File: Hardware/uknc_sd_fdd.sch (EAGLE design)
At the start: 21 parts, among them U1 USD-SOCKET

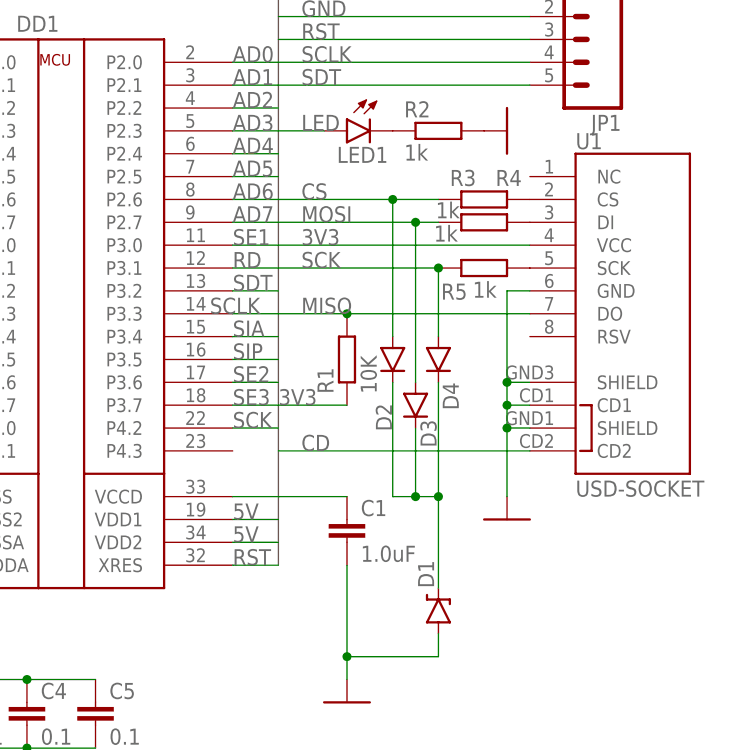
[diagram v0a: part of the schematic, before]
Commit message: исправлена схема
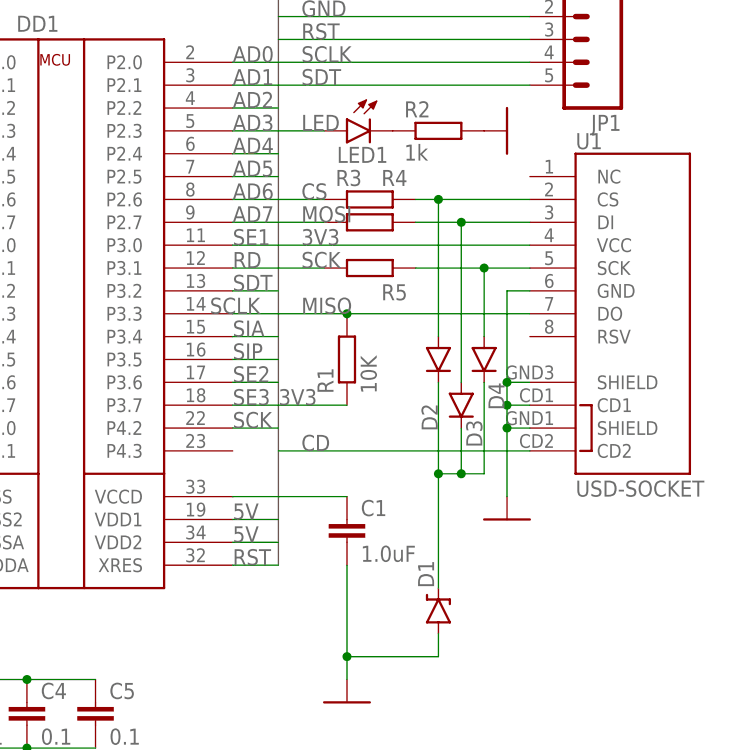
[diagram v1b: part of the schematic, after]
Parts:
- R3, R4, R5: value 1k -> (none)
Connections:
- net CS: no longer D2.A
- net MOSI: no longer D3.A
- net N$4: now also D2.A, R3.2, U1.CS; no longer R5.2, U1.SCK
- net N$5: now also D3.A
- net N$6: now also D4.A, R5.2, U1.SCK; no longer R3.2, U1.CS
- net SCK: no longer D4.A
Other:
- moved on the sheet: D2, D3, D4, R3, R4, R5
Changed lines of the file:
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@@
 <setting verticaltext="up"/>
 </settings>
-<grid distance="0.1" unitdist="inch" unit="inch" style="lines" multiple="1" display="no" altdistance="0.000000123031" altunitdist="inch" altunit="inch"/>
+<grid distance="0.1" unitdist="inch" unit="inch" style="lines" multiple="1" display="no" altdistance="0.01" altunitdist="inch" altunit="inch"/>
 <layers>
 <layer number="1" name="Top" color="4" fill="1" visible="no" active="no"/>
@@
 <part name="C5" library="resistor" deviceset="C-EU" device="C0805" value="0.1"/>
 <part name="C6" library="resistor" deviceset="CPOL-EU" device="E1.8-4" value="10.0"/>
-<part name="R3" library="resistor" deviceset="R-EU_" device="R0805" value="1k"/>
-<part name="R4" library="resistor" deviceset="R-EU_" device="R0805" value="1k"/>
-<part name="R5" library="resistor" deviceset="R-EU_" device="R0805" value="1k"/>
+<part name="R3" library="resistor" deviceset="R-EU_" device="R0805"/>
+<part name="R4" library="resistor" deviceset="R-EU_" device="R0805"/>
+<part name="R5" library="resistor" deviceset="R-EU_" device="R0805"/>
 </parts>
 <sheets>
@@
 <instance part="JP1" gate="G$1" x="132.08" y="91.44" rot="R180"/>
 <instance part="U$8" gate="G$1" x="121.92" y="38.1"/>
-<instance part="D2" gate="G$1" x="109.22" y="55.88" smashed="yes" rot="R270">
-<attribute name="NAME" x="107.35603125" y="50.992" size="1.778" layer="95" rot="R270"/>
-<attribute name="VALUE" x="106.9086" y="53.34" size="1.778" layer="96" rot="R270"/>
+<instance part="D2" gate="G$1" x="114.3" y="55.88" smashed="yes" rot="R270">
+<attribute name="NAME" x="112.43603125" y="50.992" size="1.778" layer="95" rot="R270"/>
+<attribute name="VALUE" x="111.9886" y="53.34" size="1.778" layer="96" rot="R270"/>
 </instance>
-<instance part="D3" gate="G$1" x="111.76" y="50.8" smashed="yes" rot="R270">
-<attribute name="NAME" x="112.31370625" y="49.184971875" size="1.778" layer="95" rot="R270"/>
-<attribute name="VALUE" x="109.4486" y="48.26" size="1.778" layer="96" rot="R270"/>
+<instance part="D3" gate="G$1" x="116.84" y="50.8" smashed="yes" rot="R270">
+<attribute name="NAME" x="117.39370625" y="49.184971875" size="1.778" layer="95" rot="R270"/>
+<attribute name="VALUE" x="114.5286" y="48.26" size="1.778" layer="96" rot="R270"/>
 </instance>
-<instance part="D4" gate="G$1" x="114.3" y="55.88" rot="R270"/>
+<instance part="D4" gate="G$1" x="119.38" y="55.88" rot="R270"/>
 <instance part="R2" gate="G$1" x="114.3" y="81.28"/>
 <instance part="U$9" gate="G$1" x="121.92" y="81.28" rot="R90"/>
@@
 <instance part="C5" gate="G$1" x="76.2" y="17.78"/>
 <instance part="C6" gate="G$1" x="33.02" y="12.7"/>
-<instance part="R3" gate="G$1" x="119.38" y="73.66" smashed="yes">
-<attribute name="NAME" x="115.57" y="75.1586" size="1.778" layer="95"/>
-<attribute name="VALUE" x="114.00561875" y="71.567578125" size="1.778" layer="96"/>
+<instance part="R3" gate="G$1" x="106.68" y="73.66"/>
+<instance part="R4" gate="G$1" x="106.68" y="71.12" smashed="yes">
+<attribute name="NAME" x="107.95" y="75.1586" size="1.778" layer="95"/>
+<attribute name="VALUE" x="102.87" y="67.818" size="1.778" layer="96"/>
 </instance>
-<instance part="R4" gate="G$1" x="119.38" y="71.12" smashed="yes">
-<attribute name="NAME" x="120.65" y="75.1586" size="1.778" layer="95"/>
-<attribute name="VALUE" x="113.79229375" y="68.977884375" size="1.778" layer="96"/>
-</instance>
-<instance part="R5" gate="G$1" x="119.38" y="66.04" smashed="yes">
-<attribute name="NAME" x="114.59438125" y="62.52975" size="1.778" layer="95"/>
-<attribute name="VALUE" x="118.11" y="62.738" size="1.778" layer="96"/>
+<instance part="R5" gate="G$1" x="106.68" y="66.04" smashed="yes">
+<attribute name="NAME" x="107.95" y="62.4586" size="1.778" layer="95"/>
+<attribute name="VALUE" x="102.87" y="62.738" size="1.778" layer="96"/>
 </instance>
 </instances>
@@
 <label x="99.06" y="73.66" size="1.778" layer="95"/>
 <pinref part="R3" gate="G$1" pin="1"/>
-<wire x1="114.3" y1="73.66" x2="109.22" y2="73.66" width="0.1524" layer="91"/>
-<pinref part="D2" gate="G$1" pin="A"/>
-<wire x1="109.22" y1="73.66" x2="96.52" y2="73.66" width="0.1524" layer="91"/>
-<wire x1="109.22" y1="58.42" x2="109.22" y2="73.66" width="0.1524" layer="91"/>
-<junction x="109.22" y="73.66"/>
+<wire x1="101.6" y1="73.66" x2="96.52" y2="73.66" width="0.1524" layer="91"/>
 </segment>
 </net>
@@
 <label x="99.06" y="71.12" size="1.778" layer="95"/>
 <pinref part="R4" gate="G$1" pin="1"/>
-<wire x1="114.3" y1="71.12" x2="111.76" y2="71.12" width="0.1524" layer="91"/>
-<pinref part="D3" gate="G$1" pin="A"/>
-<wire x1="111.76" y1="71.12" x2="96.52" y2="71.12" width="0.1524" layer="91"/>
-<wire x1="111.76" y1="53.34" x2="111.76" y2="71.12" width="0.1524" layer="91"/>
-<junction x="111.76" y="71.12"/>
+<wire x1="101.6" y1="71.12" x2="96.52" y2="71.12" width="0.1524" layer="91"/>
 </segment>
 </net>
@@
 <label x="99.06" y="66.04" size="1.778" layer="95"/>
 <pinref part="R5" gate="G$1" pin="1"/>
-<wire x1="114.3" y1="66.04" x2="96.52" y2="66.04" width="0.1524" layer="91"/>
-<pinref part="D4" gate="G$1" pin="A"/>
-<wire x1="114.3" y1="58.42" x2="114.3" y2="66.04" width="0.1524" layer="91"/>
-<junction x="114.3" y="66.04"/>
+<wire x1="101.6" y1="66.04" x2="96.52" y2="66.04" width="0.1524" layer="91"/>
 </segment>
 </net>
@@
 <net name="N$2" class="0">
 <segment>
+<pinref part="D1" gate="G$1" pin="C"/>
 <pinref part="D2" gate="G$1" pin="C"/>
-<wire x1="109.22" y1="53.34" x2="109.22" y2="40.64" width="0.1524" layer="91"/>
+<wire x1="114.3" y1="30.48" x2="114.3" y2="43.18" width="0.1524" layer="91"/>
 <pinref part="D3" gate="G$1" pin="C"/>
-<wire x1="111.76" y1="48.26" x2="111.76" y2="40.64" width="0.1524" layer="91"/>
-<wire x1="109.22" y1="40.64" x2="111.76" y2="40.64" width="0.1524" layer="91"/>
+<wire x1="114.3" y1="43.18" x2="114.3" y2="53.34" width="0.1524" layer="91"/>
+<wire x1="116.84" y1="48.26" x2="116.84" y2="43.18" width="0.1524" layer="91"/>
+<wire x1="116.84" y1="43.18" x2="114.3" y2="43.18" width="0.1524" layer="91"/>
+<junction x="114.3" y="43.18"/>
 <pinref part="D4" gate="G$1" pin="C"/>
-<wire x1="114.3" y1="53.34" x2="114.3" y2="40.64" width="0.1524" layer="91"/>
-<pinref part="D1" gate="G$1" pin="C"/>
-<wire x1="114.3" y1="40.64" x2="114.3" y2="30.48" width="0.1524" layer="91"/>
-<wire x1="111.76" y1="40.64" x2="114.3" y2="40.64" width="0.1524" layer="91"/>
-<junction x="111.76" y="40.64"/>
-<junction x="114.3" y="40.64"/>
+<wire x1="119.38" y1="53.34" x2="119.38" y2="43.18" width="0.1524" layer="91"/>
+<wire x1="119.38" y1="43.18" x2="116.84" y2="43.18" width="0.1524" layer="91"/>
+<junction x="116.84" y="43.18"/>
 </segment>
 </net>
@@
 <net name="N$4" class="0">
 <segment>
+<pinref part="R3" gate="G$1" pin="2"/>
+<pinref part="U1" gate="G$1" pin="CS"/>
+<wire x1="111.76" y1="73.66" x2="114.3" y2="73.66" width="0.1524" layer="91"/>
+<pinref part="D2" gate="G$1" pin="A"/>
+<wire x1="114.3" y1="73.66" x2="124.46" y2="73.66" width="0.1524" layer="91"/>
+<wire x1="114.3" y1="58.42" x2="114.3" y2="73.66" width="0.1524" layer="91"/>
+<junction x="114.3" y="73.66"/>
+</segment>
+</net>
+<net name="N$5" class="0">
+<segment>
+<pinref part="R4" gate="G$1" pin="2"/>
+<pinref part="U1" gate="G$1" pin="DI"/>
+<wire x1="111.76" y1="71.12" x2="116.84" y2="71.12" width="0.1524" layer="91"/>
+<pinref part="D3" gate="G$1" pin="A"/>
+<wire x1="116.84" y1="71.12" x2="124.46" y2="71.12" width="0.1524" layer="91"/>
+<wire x1="116.84" y1="53.34" x2="116.84" y2="71.12" width="0.1524" layer="91"/>
+<junction x="116.84" y="71.12"/>
+</segment>
+</net>
+<net name="N$6" class="0">
+<segment>
+<pinref part="R5" gate="G$1" pin="2"/>
 <pinref part="U1" gate="G$1" pin="SCK"/>
-<pinref part="R5" gate="G$1" pin="2"/>
-</segment>
-</net>
-<net name="N$5" class="0">
-<segment>
-<pinref part="U1" gate="G$1" pin="DI"/>
-<pinref part="R4" gate="G$1" pin="2"/>
-</segment>
-</net>
-<net name="N$6" class="0">
-<segment>
-<pinref part="U1" gate="G$1" pin="CS"/>
-<pinref part="R3" gate="G$1" pin="2"/>
-</segment>
-</net>
+<wire x1="111.76" y1="66.04" x2="119.38" y2="66.04" width="0.1524" layer="91"/>
+<pinref part="D4" gate="G$1" pin="A"/>
+<wire x1="119.38" y1="66.04" x2="124.46" y2="66.04" width="0.1524" layer="91"/>
+<wire x1="119.38" y1="58.42" x2="119.38" y2="66.04" width="0.1524" layer="91"/>
+<junction x="119.38" y="66.04"/>
+</segment>
+</net>
